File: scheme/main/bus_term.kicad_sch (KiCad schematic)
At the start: 1 part, among them J2 Conn_01x03

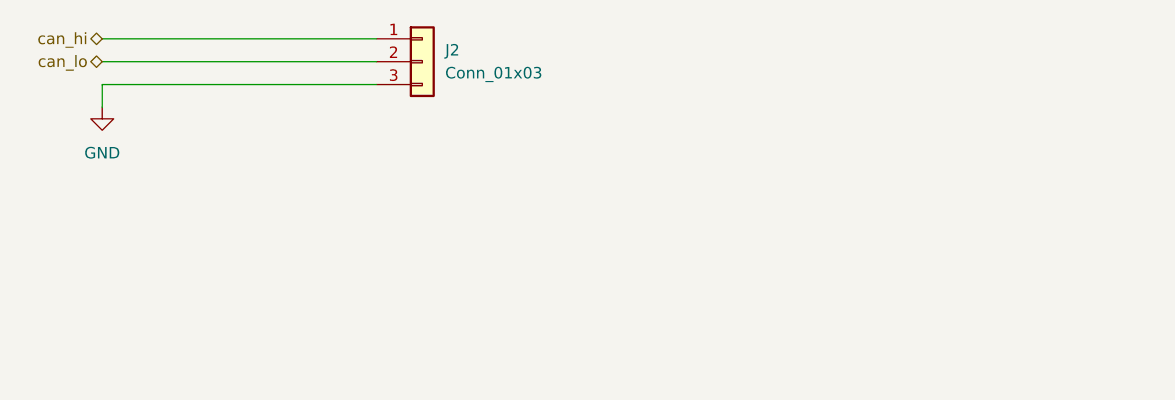
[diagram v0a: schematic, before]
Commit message: boards schematic sheets & more
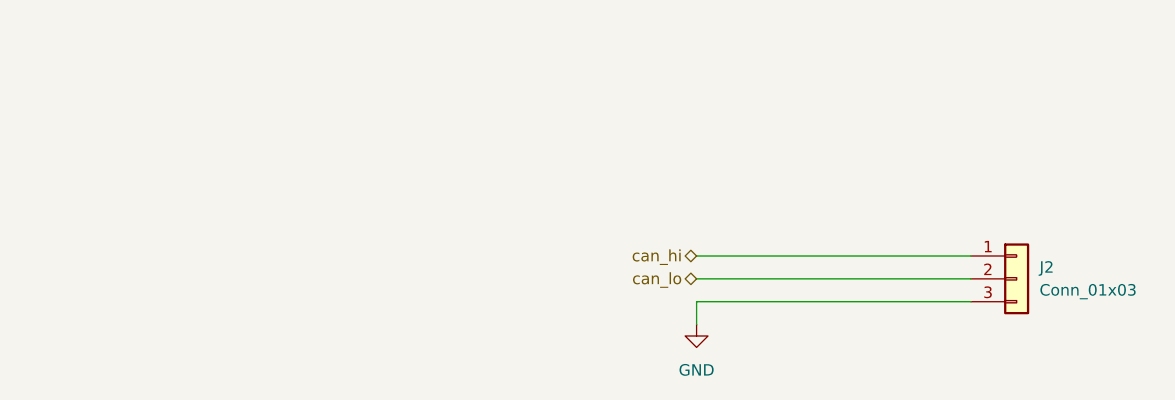
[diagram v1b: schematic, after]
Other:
- moved on the sheet: J2
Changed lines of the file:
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@@
 	(wire
 		(pts
-			(xy 62.23 72.39) (xy 92.71 72.39)
+			(xy 128.27 96.52) (xy 158.75 96.52)
 		)
 		(stroke
@@
 	(wire
 		(pts
-			(xy 62.23 74.93) (xy 62.23 72.39)
+			(xy 128.27 99.06) (xy 128.27 96.52)
 		)
 		(stroke
@@
 	(wire
 		(pts
-			(xy 62.23 67.31) (xy 92.71 67.31)
+			(xy 128.27 91.44) (xy 158.75 91.44)
 		)
 		(stroke
@@
 	(wire
 		(pts
-			(xy 62.23 69.85) (xy 92.71 69.85)
+			(xy 128.27 93.98) (xy 158.75 93.98)
 		)
 		(stroke
@@
 	(hierarchical_label "can_hi"
 		(shape bidirectional)
-		(at 62.23 67.31 180)
+		(at 128.27 91.44 180)
 		(fields_autoplaced yes)
 		(effects
@@
 	(hierarchical_label "can_lo"
 		(shape bidirectional)
-		(at 62.23 69.85 180)
+		(at 128.27 93.98 180)
 		(fields_autoplaced yes)
 		(effects
@@
 	(symbol
 		(lib_id "Connector_Generic:Conn_01x03")
-		(at 97.79 69.85 0)
+		(at 163.83 93.98 0)
 		(unit 1)
 		(exclude_from_sim no)
@@
 		(fields_autoplaced yes)
 		(property "Reference" "J2"
-			(at 100.33 68.5799 0)
+			(at 166.37 92.7099 0)
 			(effects
 				(font
@@
 		)
 		(property "Value" "Conn_01x03"
-			(at 100.33 71.1199 0)
+			(at 166.37 95.2499 0)
 			(effects
 				(font
@@
 		)
 		(property "Footprint" ""
-			(at 97.79 69.85 0)
+			(at 163.83 93.98 0)
 			(effects
 				(font
@@
 		)
 		(property "Datasheet" "~"
-			(at 97.79 69.85 0)
+			(at 163.83 93.98 0)
 			(effects
 				(font
@@
 		)
 		(property "Description" "Generic connector, single row, 01x03, script generated (kicad-library-utils/schlib/autogen/connector/)"
-			(at 97.79 69.85 0)
+			(at 163.83 93.98 0)
 			(effects
 				(font
@@
 	(symbol
 		(lib_id "power:GND")
-		(at 62.23 74.93 0)
+		(at 128.27 99.06 0)
 		(unit 1)
 		(exclude_from_sim no)
@@
 		(fields_autoplaced yes)
 		(property "Reference" "#PWR0111"
-			(at 62.23 81.28 0)
+			(at 128.27 105.41 0)
 			(effects
 				(font
@@
 		)
 		(property "Value" "GND"
-			(at 62.23 80.01 0)
+			(at 128.27 104.14 0)
 			(effects
 				(font
@@
 		)
 		(property "Footprint" ""
-			(at 62.23 74.93 0)
+			(at 128.27 99.06 0)
 			(effects
 				(font
@@
 		)
 		(property "Datasheet" ""
-			(at 62.23 74.93 0)
+			(at 128.27 99.06 0)
 			(effects
 				(font
@@
 		)
 		(property "Description" "Power symbol creates a global label with name \"GND\" , ground"
-			(at 62.23 74.93 0)
+			(at 128.27 99.06 0)
 			(effects
 				(font
